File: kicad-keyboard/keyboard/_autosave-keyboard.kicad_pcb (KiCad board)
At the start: 2 copper layers, 149.1 x 131.9 mm, 96 parts, among them SW1 SW_Push, SW10 SW_Push, SW11 SW_Push, SW12 SW_Push, SW13 SW_Push, SW14 SW_Push, SW15 SW_Push, SW16 SW_Push, SW17 SW_Push, SW18 SW_Push, SW19 SW_Push, SW2 SW_Push, SW20 SW_Push, SW21 SW_Push, SW22 SW_Push, SW23 SW_Push, SW24 SW_Push, SW25 SW_Push, SW26 SW_Push, SW27 SW_Push, SW28 SW_Push, SW29 SW_Push, SW3 SW_Push, SW30 SW_Push, SW31 SW_Push, SW32 SW_Push, SW33 SW_Push, SW34 SW_Push, SW35 SW_Push, SW36 SW_Push, SW37 SW_Push, SW38 SW_Push, SW39 SW_Slide_DPDT, SW4 SW_Push, SW5 SW_Push, SW6 SW_Push, SW7 SW_Push, SW8 SW_Push, SW9 SW_Push

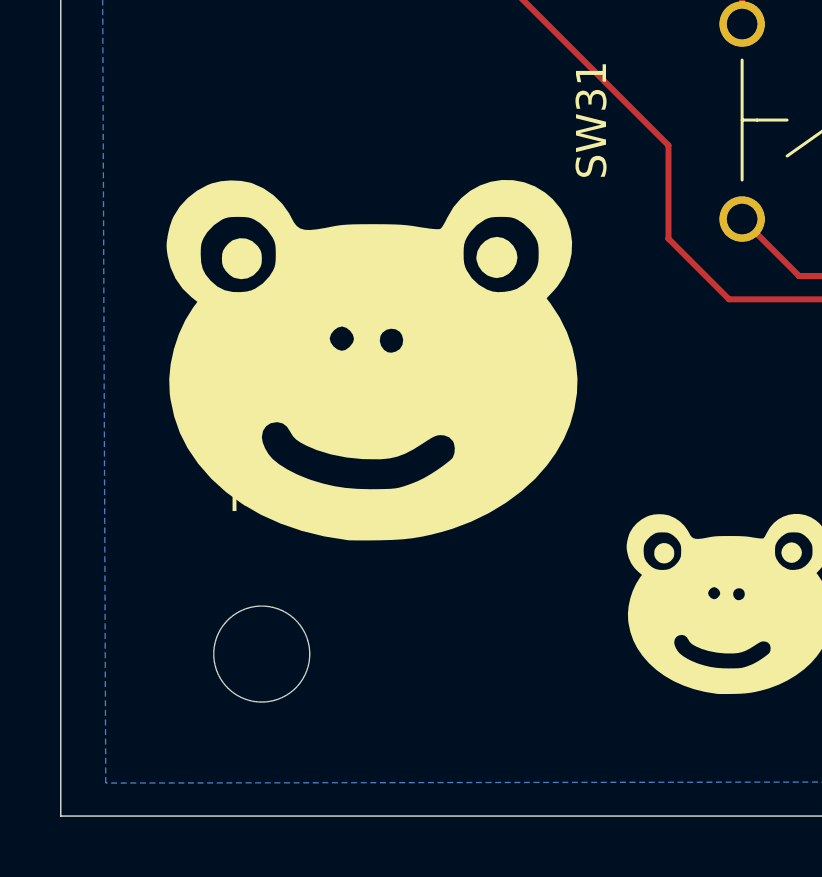
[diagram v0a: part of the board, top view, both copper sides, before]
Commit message: kicad = misogyne
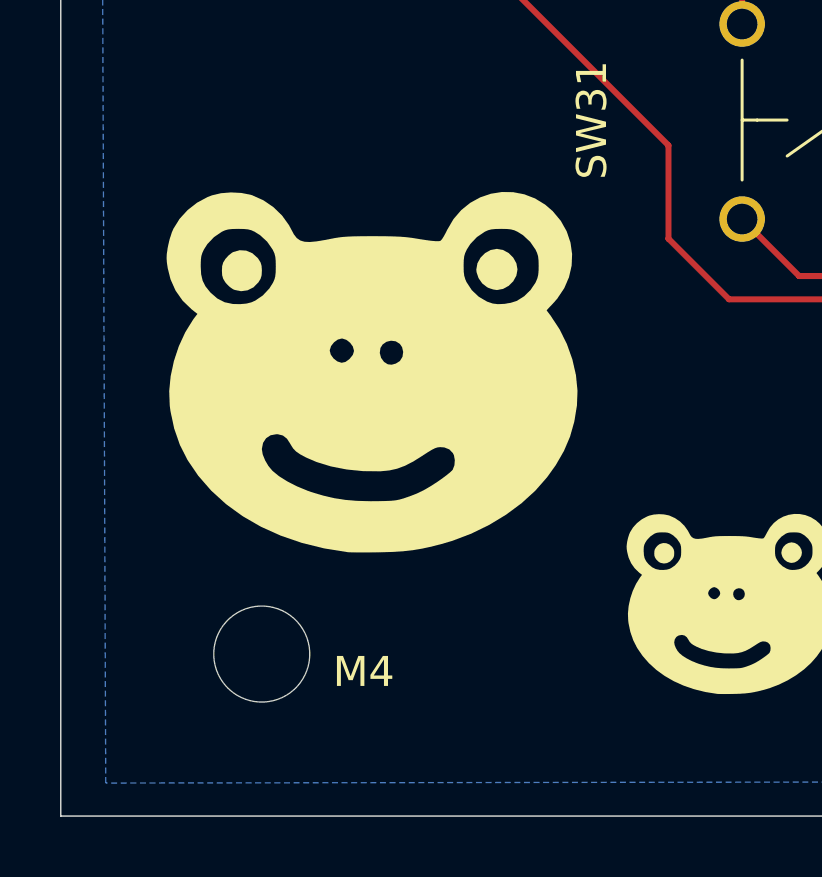
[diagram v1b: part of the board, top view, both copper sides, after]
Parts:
- moved G*** 0.40 mm to (50.1, 161.4)
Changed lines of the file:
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@@
 	(footprint "LOGO"
 		(layer "F.Cu")
-		(at 50.122144 160.951857)
+		(at 50.122144 161.351857)
 		(property "Reference" "G***"
 			(at 0 0 0)
@@
 		(at 29.12 155.47)
 		(property "Reference" "M4"
-			(at 0 -0.5 0)
+			(at 3.48 5.33 0)
 			(unlocked yes)
 			(layer "F.SilkS")
